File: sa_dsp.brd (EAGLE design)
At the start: 2 parts, among them U1 10CL016YF484C6G, U2 OSD3358-512M-BSM

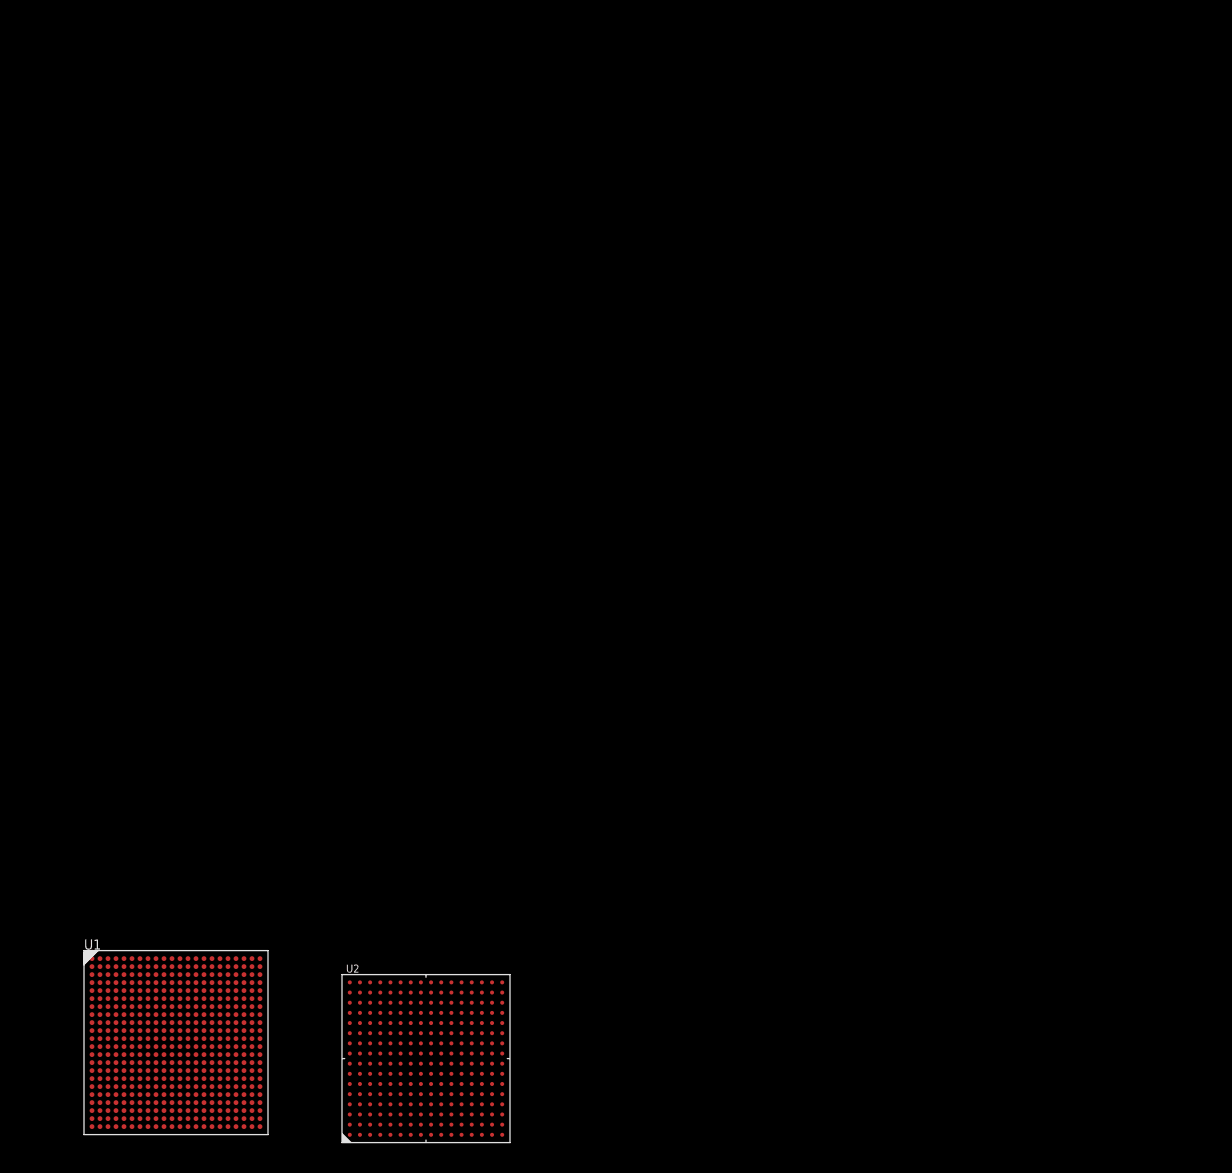
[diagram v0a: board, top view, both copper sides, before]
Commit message: Work on the DSP
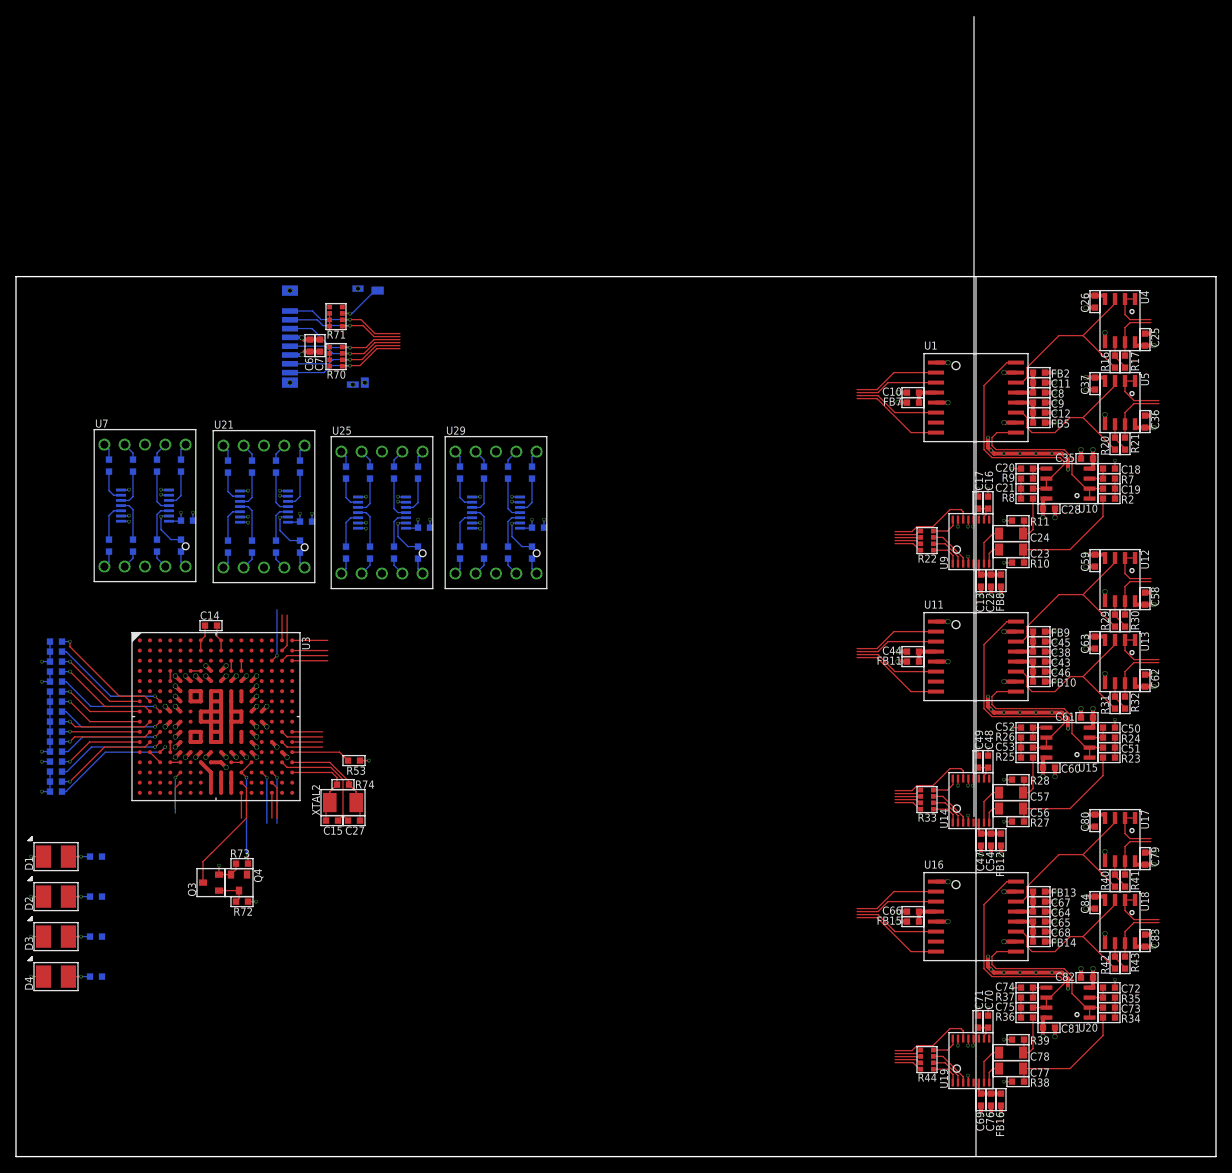
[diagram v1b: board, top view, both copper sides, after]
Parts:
- removed U2: OSD3358-512M-BSM, Octavo-Systems:OSD335X-BGA-256
- added C10, C13, C14, C17, C2, C25, C26, C28, C3, C30, C35, C36, C37, C38, C43, C44, C47, C49, C5, C58, C59, C6, C60, C61, C62, C63, C64, C65, C66, C69, C71, C79, C8, C80, C81, C82, C83, C84, C9: 100nF 16V, CAPACITORS:0603
- added C11, C12, C16, C22, C45, C46, C48, C54, C67, C68, C7, C70, C76: 10uF 10V, CAPACITORS:0603
- added C15, C27: 15pF 50V, CAPACITORS:0603
- added C18, C19, C20, C21, C50, C51, C52, C53, C72, C73, C74, C75: 470pF 16V, CAPACITORS:0603
- added C23, C24, C56, C57, C77, C78: 330nF 16V, CAPACITORS:1206
- added CN1: uSD, CONNECTORs:114-00841-68
- added D1, D2, D3, D4: RED STATUS, OPTO:VLMT3100
- added FB10, FB11, FB12, FB13, FB14, FB15, FB16, FB2, FB5, FB7, FB8, FB9: 600R, INDUCTORS:0603
- added Q3, Q4: 2N7002, TRANSISTORs:SOT23-3
- added R10, R11, R27, R28, R38, R39: 180k, r_0603:0603
- added R108, R109, R110, R111, R112, R113, R114, R115, R18, R19, R45, R46, R47, R48, R49, R50, R51, R52, R6, R78, R79, R80, R82, R83, R92, R93, R94, R95, R96, R97, R98, R99: 470R, r_0603:0603
- added R16, R17, R20, R21, R29, R30, R31, R32, R40, R41, R42, R43, R75, R76, R77, R81: 1.0k, r_0603:0603
- added R2, R23, R24, R25, R26, R34, R35, R36, R37, R7, R8, R9: 20k, r_0603:0603
- added R22, R33, R44: 22R, RESISTORS:1206_ARRAY
- added R53: 10k, r_0603:0603
- added R54, R55, R56, R57, R58, R59, R60, R61, R62, R63, R64, R65, R66, R67, R68, R69: 100k, r_0603:0603
- added R70, R71: 10k, RESISTORS:1206_ARRAY
- added R72, R73, R74: 1.0M, r_0603:0603
- added U10, U12, U13, U15, U17, U18, U20, U4, U5: LME49720, ICs:SO8
- added U11, U16: PGA2311, ICs:SOL16
- added U14, U19, U9: PCM1754, ICs:SSOP16-4MM
- added U21, U25, U29, U7: 7 SEG, OPTO:SC56-11SURKWA
- added U22, U26, U30, U8: 74HC164A, ICs:SSOP14-4.5MM
- added U3: OSD3358-512M-BSM, Octavo-Systems:OSD335X-BGA-256
- added XTAL2: 24MHz, CRYSTALS:5X3.2SMD
- U1: value 10CL016YF484C6G -> PGA2311; device ICs:FBGA484 -> ICs:SOL16
- moved U1 128.5 mm to (120.0, 94.9)
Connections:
- removed net SYS_RTC_1P8V: U2.K11, U2.L11
- removed net SYS_VDD1_3P3V: U2.F6, U2.F7, U2.G6, U2.G7
- removed net SYS_VDD2_3P3V: U2.F11, U2.G11
- removed net SYS_VDD3_3P3V: U2.F8, U2.G8, U2.H7, U2.H8, U2.J7, U2.J8, U2.K8, U2.L8
- removed net SYS_VDD_1P8V: U2.F10, U2.G10, U2.H10, U2.H11, U2.J10, U2.J11, U2.K10, U2.L10
- removed net SYS_VOUT: U2.K6, U2.K7, U2.L6, U2.L7
- removed net VDDSHV1: U2.J9
- removed net VDDSHV2: U2.K9
- removed net VDDSHV3: U2.L9
- removed net VDDSHV4: U2.F9
- removed net VDDSHV5: U2.G9
- removed net VDDSHV6: U2.H9
- removed net VIN_AC: U2.P10, U2.R10, U2.T10
- removed net VIN_BAT: U2.P8, U2.R8, U2.T8
- removed net VIN_USB: U2.P9, U2.R9, U2.T9
- new net +5V: C25.2, C28.2, C36.2, C58.2, C60.2, C62.2, C79.2, C81.2, C83.2, FB10.1, FB12.2, FB14.1, FB16.2, FB5.1, FB8.2, U10.8, U12.8, U13.8, U15.8, U17.8, U18.8, U20.8, U4.8, U5.8
- new net -5V: C26.1, C35.1, C37.1, C59.1, C61.1, C63.1, C80.1, C82.1, C84.1, FB13.1, FB2.1, FB9.1, U10.4, U12.4, U13.4, U15.4, U17.4, U18.4, U20.4, U4.4, U5.4
- new net 3V3: C2.2, C3.2, C30.2, C5.2, C6.2, C7.2, CN1.4, R54.2, R55.2, R56.2, R70.5, R70.6, R70.7, R70.8, R71.6, R71.7, R71.8, R72.2, U22.14, U22.9, U26.14, U26.9, U30.14, U30.9, U8.14, U8.9
- new net 5V: FB11.2, FB15.2, FB7.2, U1.1, U11.1, U16.1, U3.M15, U3.P10, U3.R10, U3.T10
- new net 5VUSB: U3.J16
- new net AGND: C11.1, C12.1, C13.1, C16.1, C17.1, C18.2, C20.2, C22.1, C25.1, C26.2, C28.1, C35.2, C36.1, C37.2, C38.1, C43.1, C45.1, C46.1, C47.1, C48.1, C49.1, C50.2, C52.2, C54.1, C58.1, C59.2, C60.1, C61.2, C62.1, C63.2, C64.1, C65.1, C67.1, C68.1, C69.1, C70.1, C71.1, C72.2, C74.2, C76.1, C79.1, C8.1, C80.2, C81.1, C82.2, C83.1, C84.2, C9.1, R10.1, R11.1, R27.1, R28.1, R38.1, R39.1, U1.10, U1.15, U11.10, U11.15, U12.5, U13.5, U14.9, U16.10, U16.15, U17.5, U18.5, U19.9, U4.5, U5.5, U9.9
- new net AM_DEBUG_UART_RX: U3.A12
- new net AM_DEBUG_UART_TX: U3.B12
- new net AM_EEPROM_WP: U3.M2, U3.N3
- new net AM_PMIC_PGOOD: Q4.1, R73.2, U3.N12, U3.P11
- new net AM_PWR_BTN: U3.T11
- new net AM_STM_NRST: U3.P5
- new net AM_USR_LED0: R75.1, U3.P13
- new net AM_USR_LED1: R76.1, U3.T14
- new net AM_USR_LED2: R77.1, U3.R14
- new net AM_USR_LED3: R81.1, U3.P14
- new net AM_WARM_!RST: Q3.2, U3.R11
- new net DAC0_I2S_BCLK: R22.8, R33.8, R44.8
- new net DAC0_I2S_DATA: R22.7, R33.7, R44.7
- new net DAC0_I2S_LRCLK: R22.6, R33.6, R44.6
- new net DAC0_I2S_SCLK: R22.5, R33.5, R44.5
- new net DAC_MUTE: U14.14, U19.14, U9.14
- new net DISP_SPI_!CE: U22.2, U26.2, U30.2, U8.2
- new net DISP_SPI_MOSI: U22.1, U26.1, U30.1, U8.1
- new net DISP_SPI_SCLK: U22.8, U26.8, U30.8, U8.8
- new net GND: C10.1, C2.1, C3.1, C30.1, C44.1, C5.1, C6.1, C66.1, C7.1, CN1.6, CN1.CD_2, CN1.MNT1, CN1.MNT2, CN1.MNT3, CN1.MNT4, D1.K, D2.K, D3.K, D4.K, Q3.3, Q4.3, R53.1, R57.1, R58.1, R59.1, R60.1, R61.1, R62.1, R63.1, R64.1, R65.1, R66.1, R67.1, R68.1, R69.1, R73.1, U1.5, U11.5, U14.12, U14.13, U14.15, U14.4, U16.5, U19.12, U19.13, U19.15, U19.4, U21.3, U21.8, U22.7, U25.3, U25.8, U26.7, U29.3, U29.8, U3.D8, U3.D9, U3.E10, U3.E11, U3.E12, U3.E5, U3.E6, U3.E7, U3.E8, U3.E9, U3.F12, U3.F5, U3.G12, U3.G5, U3.H12, U3.H13, U3.H4, U3.H5, U3.J12, U3.J13, U3.J4, U3.J5, U3.K12, U3.K5, U3.L12, U3.L14, U3.L5, U3.M10, U3.M11, U3.M12, U3.M5, U3.M6, U3.M7, U3.M8, U3.M9, U3.N8, U3.N9, U30.7, U7.3, U7.8, U8.7, U9.12, U9.13, U9.15, U9.4
- new net MMC0_CD: CN1.CS_1, R71.3, U3.C14
- new net MMC0_CLK: CN1.5, R70.3, U3.B15
- new net MMC0_CMD: CN1.3, R70.4, U3.B16
- new net MMC0_D0: CN1.7, R70.2, U3.A16
- new net MMC0_D1: CN1.8, R70.1, U3.A15
- new net MMC0_D2: CN1.1, R71.2, U3.C16
- new net MMC0_D3: CN1.2, R71.1, U3.C15
- new net N$100: R41.2, U17.7
- new net N$101: C78.2, R36.1, R39.2
- new net N$102: C77.2, R34.1, R38.2
- new net N$103: R44.1, U19.1
- new net N$104: R44.2, U19.2
- new net N$105: R44.4, U19.16
- new net N$106: R44.3, U19.3
- new net N$107: C77.1, U19.8
- new net N$108: R40.1, U16.14, U17.3
- new net N$109: R19.1, U8.12
- new net N$11: C10.2, FB7.1, U1.4
- new net N$110: R6.1, U8.11
- new net N$111: R18.1, U8.10
- new net N$112: R50.2, U21.7
- new net N$113: R51.2, U21.6
- new net N$114: R52.2, U21.4
- new net N$115: R78.2, U21.2
- new net N$116: R79.1, U21.5
- new net N$117: R80.1, U21.10
- new net N$118: R82.1, U21.9
- new net N$119: R83.1, U21.1
- new net N$12: U4.1, U4.2
- new net N$120: R80.2, U22.6
- new net N$121: R82.2, U22.5
- new net N$122: R83.2, U22.3
- new net N$123: R78.1, U22.4
- new net N$124: U3.K6, U3.K7, U3.L6, U3.L7
- new net N$125: U3.F6, U3.F7, U3.G6, U3.G7
- new net N$126: U3.F11, U3.G11
- new net N$127: U3.K11, U3.L11
- new net N$128: U3.F8, U3.F9, U3.G8, U3.G9, U3.H7, U3.H8, U3.H9, U3.J7, U3.J8, U3.J9, U3.K8, U3.K9, U3.L8, U3.L9
- new net N$129: U3.F10, U3.G10, U3.H10, U3.H11, U3.J10, U3.J11, U3.K10, U3.L10
- new net N$13: R16.2, R17.1, U4.6
- new net N$130: U3.N10, U3.N11
- new net N$131: U3.N4, U3.N5
- new net N$132: U3.L4, U3.M4
- new net N$133: U3.D4, U3.E4
- new net N$134: U3.C10, U3.D10
- new net N$135: U3.C11, U3.D11
- new net N$136: R53.2, U3.M16
- new net N$137: R57.2, U3.G3
- new net N$138: R58.2, U3.G2
- new net N$139: R59.2, U3.G1
- new net N$140: R54.1, U3.H3
- new net N$141: R55.1, U3.H2
- new net N$142: R60.2, U3.H1
- new net N$143: R61.2, U3.J3
- new net N$144: R62.2, U3.J2
- new net N$145: R63.2, U3.J1
- new net N$146: R64.2, U3.K3
- new net N$147: R65.2, U3.K2
- new net N$148: R66.2, U3.K1
- new net N$149: R67.2, U3.L3
- new net N$150: R68.2, U3.L2
- new net N$151: R56.1, U3.L1
- new net N$152: R69.2, U3.M3
- new net N$153: U3.P9, U3.R9, U3.T9
- new net N$154: U3.N7, U3.P8, U3.R8, U3.T8
- new net N$155: C14.2, U3.A7, U3.B7
- new net N$156: C14.1, U3.A9, U3.B9
- new net N$157: Q3.1, Q4.2, R72.1
- new net N$158: C27.2, R74.1, U3.N16, XTAL2.2
- new net N$159: C15.2, R74.2, U3.P16, XTAL2.1
- new net N$160: C15.1, C27.1, U3.N15
- new net N$161: U3.D6, U3.D7
- new net N$162: D1.A, R75.2
- new net N$163: D2.A, R76.2
- new net N$164: D3.A, R77.2
- new net N$165: D4.A, R81.2
- new net N$166: R52.1, U22.12
- new net N$167: R50.1, U22.11
- new net N$168: R51.1, U22.10
- new net N$17: U5.1, U5.2
- new net N$184: R92.2, U25.7
- new net N$185: R93.2, U25.6
- new net N$186: R94.2, U25.4
- new net N$187: R95.2, U25.2
- new net N$188: R96.1, U25.5
- new net N$189: R97.1, U25.10
- new net N$190: R98.1, U25.9
- new net N$191: R99.1, U25.1
- new net N$192: R97.2, U26.6
- new net N$193: R98.2, U26.5
- new net N$194: R99.2, U26.3
- new net N$195: R95.1, U26.4
- new net N$196: R94.1, U26.12
- new net N$197: R92.1, U26.11
- new net N$198: R93.1, U26.10
- new net N$214: R108.2, U29.7
- new net N$215: R109.2, U29.6
- new net N$216: R110.2, U29.4
- new net N$217: R111.2, U29.2
- new net N$218: R112.1, U29.5
- new net N$219: R113.1, U29.10
- new net N$22: R6.2, U7.7
- new net N$220: R114.1, U29.9
- new net N$221: R115.1, U29.1
- new net N$222: R113.2, U30.6
- new net N$223: R114.2, U30.5
- new net N$224: R115.2, U30.3
- new net N$225: R111.1, U30.4
- new net N$226: R110.1, U30.12
- new net N$227: R108.1, U30.11
- new net N$228: R109.1, U30.10
- new net N$23: R18.2, U7.6
- new net N$24: R19.2, U7.4
- new net N$25: R45.2, U7.2
- new net N$26: R20.1, U1.11, U5.3
- new net N$27: R20.2, R21.1, U5.6
- new net N$28: R21.2, U5.7
- new net N$29: C13.2, C22.2, FB8.1, U9.6
- new net N$30: R46.1, U7.5
- new net N$31: R47.1, U7.10
- new net N$32: R48.1, U7.9
- new net N$33: R49.1, U7.1
- new net N$34: C16.2, C17.2, U9.10
- new net N$35: R47.2, U8.6
- new net N$36: C19.2, R2.2, R7.1
- new net N$37: C18.1, R7.2, U10.3
- new net N$38: R48.2, U8.5
- new net N$39: R49.2, U8.3
- new net N$40: C19.1, U1.9, U10.1, U10.2
- new net N$41: C21.2, R8.2, R9.1
- new net N$42: C20.1, R9.2, U10.5
- new net N$43: R45.1, U8.4
- new net N$44: C21.1, U1.16, U10.6, U10.7
- new net N$45: C24.1, U9.7
- new net N$46: R17.2, U4.7
- new net N$47: C24.2, R11.2, R8.1
- new net N$48: C23.2, R10.2, R2.1
- new net N$49: R22.1, U9.1
- new net N$50: R22.2, U9.2
- new net N$51: R22.4, U9.16
- new net N$52: R22.3, U9.3
- new net N$53: C23.1, U9.8
- new net N$54: R16.1, U1.14, U4.3
- new net N$55: C38.2, C45.2, FB9.2, U11.13
- new net N$56: C43.2, C46.2, FB10.2, U11.12
- new net N$57: C44.2, FB11.1, U11.4
- new net N$58: U12.1, U12.2
- new net N$59: R29.2, R30.1, U12.6
- new net N$60: U13.1, U13.2
- new net N$61: R31.1, U11.11, U13.3
- new net N$62: R31.2, R32.1, U13.6
- new net N$63: R32.2, U13.7
- new net N$64: C47.2, C54.2, FB12.1, U14.6
- new net N$65: C48.2, C49.2, U14.10
- new net N$66: C51.2, R23.2, R24.1
- new net N$67: C50.1, R24.2, U15.3
- new net N$68: C51.1, U11.9, U15.1, U15.2
- new net N$69: C53.2, R25.2, R26.1
- new net N$70: C52.1, R26.2, U15.5
- new net N$71: C53.1, U11.16, U15.6, U15.7
- new net N$72: C57.1, U14.7
- new net N$73: R30.2, U12.7
- new net N$74: C57.2, R25.1, R28.2
- new net N$75: C56.2, R23.1, R27.2
- new net N$76: R33.1, U14.1
- new net N$77: R33.2, U14.2
- new net N$78: R33.4, U14.16
- new net N$79: R33.3, U14.3
- new net N$8: C11.2, C8.2, FB2.2, U1.13
- new net N$80: C56.1, U14.8
- new net N$81: R29.1, U11.14, U12.3
- new net N$82: C64.2, C67.2, FB13.2, U16.13
- new net N$83: C65.2, C68.2, FB14.2, U16.12
- new net N$84: C66.2, FB15.1, U16.4
- new net N$85: U17.1, U17.2
- new net N$86: R40.2, R41.1, U17.6
- new net N$87: U18.1, U18.2
- new net N$88: R42.1, U16.11, U18.3
- new net N$89: R42.2, R43.1, U18.6
- new net N$9: C12.2, C9.2, FB5.2, U1.12
- new net N$90: R43.2, U18.7
- new net N$91: C69.2, C76.2, FB16.1, U19.6
- new net N$92: C70.2, C71.2, U19.10
- new net N$93: C73.2, R34.2, R35.1
- new net N$94: C72.1, R35.2, U20.3
- new net N$95: C73.1, U16.9, U20.1, U20.2
- new net N$96: C75.2, R36.2, R37.1
- new net N$97: C74.1, R37.2, U20.5
- new net N$98: C75.1, U16.16, U20.6, U20.7
- new net N$99: C78.1, U19.7
- new net PGA0_!CS: U1.2, U11.2, U16.2
- new net PGA_!MUTE: U1.8, U11.8, U16.8
- new net PGA_SCLK: U1.6, U11.6, U16.6
- new net PGA_SDI: U1.3, U11.3, U16.3
- new net SHIFT_OUT: R112.2, R46.2, R79.2, R96.2, U22.13, U26.13, U30.13, U8.13
- new net STM32_BOOT0: U3.R5
- new net STM_AM_UART_RX: U3.B11
- new net STM_AM_UART_TX: U3.A11
- new net USB0_DM: U3.K16
- new net USB0_DP: U3.K15
- new net USB0_ID: U3.K14
- new net USB1_DM: U3.L16
- new net USB1_DP: U3.L15
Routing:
- net AGND: track 0.00 -> 114.4 mm, vias 0 -> 90
- net GND: track 0.00 -> 91.4 mm, vias 0 -> 77
- net PGA_!MUTE: track 0.00 -> 34.9 mm
- net PGA_SCLK: track 0.00 -> 32.3 mm
- net PGA0_!CS: track 0.00 -> 32.3 mm
- net DAC_MUTE: track 0.00 -> 32.3 mm
- net +5V: track 0.00 -> 31.7 mm, vias 0 -> 15
- net PGA_SDI: track 0.00 -> 31.2 mm
- net N$98: track 0.00 -> 30.0 mm
- net N$71: track 0.00 -> 30.0 mm
- net N$44: track 0.00 -> 30.0 mm
- net -5V: track 0.00 -> 28.3 mm, vias 0 -> 12
- net 3V3: track 0.00 -> 28.0 mm, vias 0 -> 14
- net N$128: track 0.00 -> 24.1 mm
- net N$81: track 0.00 -> 23.9 mm
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- added copper zone on layer 3, net 3V3
- added copper zone on layer 2, net GND
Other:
- board outline added: 150 x 110 mm
